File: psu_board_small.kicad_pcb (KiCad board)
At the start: 2 copper layers, 23 parts

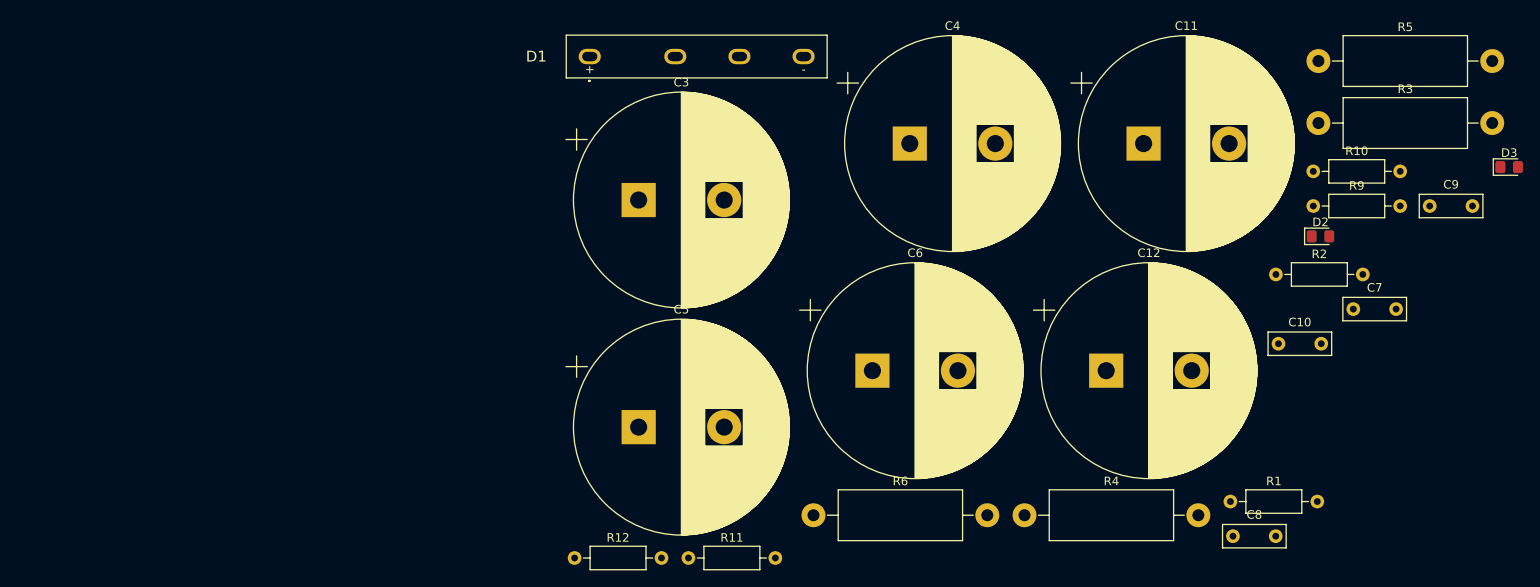
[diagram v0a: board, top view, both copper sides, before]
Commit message: finished pcb layout
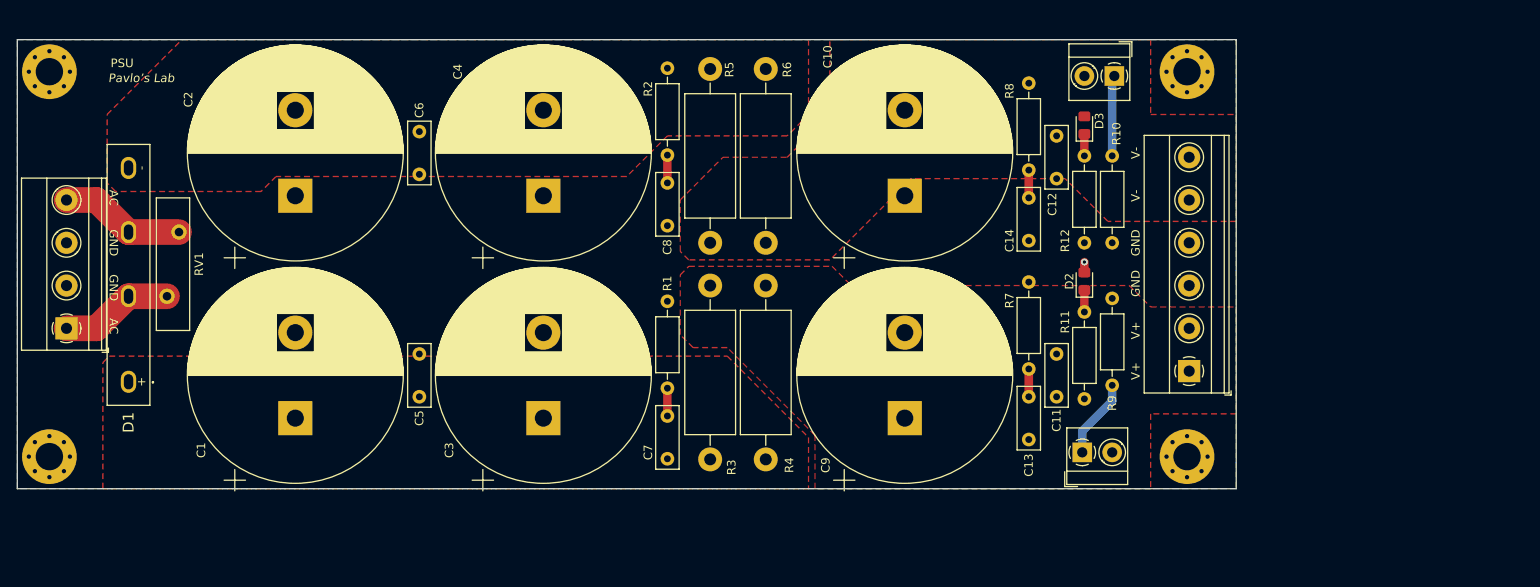
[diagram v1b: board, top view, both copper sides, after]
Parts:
- added C11: 100n, Capacitor_THT:C_Rect_L7.2mm_W2.5mm_P5.00mm_FKS2_FKP2_MKS2_MKP2, F.Cu at (144.0, 108.0)
- added C12: 100n, Capacitor_THT:C_Rect_L7.2mm_W2.5mm_P5.00mm_FKS2_FKP2_MKS2_MKP2, F.Cu at (144.0, 82.5)
- added C13: 100n, Capacitor_THT:C_Rect_L7.2mm_W2.5mm_P5.00mm_FKS2_FKP2_MKS2_MKP2, F.Cu at (140.8, 113.0)
- added C14: 100n, Capacitor_THT:C_Rect_L7.2mm_W2.5mm_P5.00mm_FKS2_FKP2_MKS2_MKP2, F.Cu at (140.8, 89.8)
- added H1: MountingHole, MountingHole:MountingHole_3.2mm_M3_Pad_Via, F.Cu at (26.2, 115.0)
- added H2: MountingHole, MountingHole:MountingHole_3.2mm_M3_Pad_Via, F.Cu at (26.2, 70.0)
- added H3: MountingHole, MountingHole:MountingHole_3.2mm_M3_Pad_Via, F.Cu at (159.2, 70.0)
- added H4: MountingHole, MountingHole:MountingHole_3.2mm_M3_Pad_Via, F.Cu at (159.2, 115.0)
- added J1: AC, TerminalBlock_Phoenix:TerminalBlock_Phoenix_MKDS-1,5-4_1x04_P5.00mm_Horizontal, F.Cu at (28.2, 100.0)
- added J2: LED, TerminalBlock_MetzConnect:TerminalBlock_MetzConnect_Type059_RT06302HBWC_1x02_P3.50mm_Horizontal, F.Cu at (147.0, 114.5)
- added J3: LED, TerminalBlock_MetzConnect:TerminalBlock_MetzConnect_Type059_RT06302HBWC_1x02_P3.50mm_Horizontal, F.Cu at (150.8, 70.5)
- added J4: DC, TerminalBlock_Phoenix:TerminalBlock_Phoenix_MKDS-1,5-6_1x06_P5.00mm_Horizontal, F.Cu at (159.5, 105.0)
- added R7: 10R, Resistor_THT:R_Axial_DIN0207_L6.3mm_D2.5mm_P10.16mm_Horizontal, F.Cu at (140.8, 104.8)
- added R8: 10R, Resistor_THT:R_Axial_DIN0207_L6.3mm_D2.5mm_P10.16mm_Horizontal, F.Cu at (140.8, 81.5)
- added RV1: MOV-14D101KTR, Varistor:RV_Disc_D15.5mm_W3.9mm_P7.5mm, F.Cu at (40.0, 96.2)
- moved C5 109.7 mm to (69.5, 108.0), turned to 90 degrees
- moved C6 104.1 mm to (69.5, 82.0), turned to 90 degrees
- moved C7 93.9 mm to (98.5, 115.2), turned to 90 degrees
- moved R5 74.2 mm to (103.5, 90.0), turned to 90 degrees
- moved R3 73.6 mm to (103.5, 95.0), turned to 270 degrees
- moved C8 72.8 mm to (98.5, 88.0), turned to 90 degrees
- moved R2 72.5 mm to (98.5, 79.8), turned to 90 degrees
- moved C2 72.1 mm to (55.0, 84.5), turned to 90 degrees
- moved D1 71.9 mm to (35.5, 92.5), turned to 90 degrees
- moved R12 70.1 mm to (147.2, 90.0), turned to 90 degrees
- moved R1 67.1 mm to (98.5, 107.0), turned to 90 degrees
- moved D3 49.9 mm to (147.2, 76.2), turned to 90 degrees
- moved R11 49.9 mm to (147.2, 108.2), turned to 90 degrees
- moved C1 47.6 mm to (55.0, 110.5), turned to 90 degrees
- moved C4 43.6 mm to (84.0, 84.5), turned to 90 degrees
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- renumbered C3 to C1, C12 to C10, C4 to C2, C5 to C3, C6 to C4, C7 to C5, C8 to C6, C9 to C7, C10 to C8, C11 to C9
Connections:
- D1 pad 2: (no net) -> /AC1
- D1 pad 3: (no net) -> /AC4
- R10 pad 2: (no net) -> Net-(J3-Pad1)
- R9 pad 2: (no net) -> Net-(J2-Pad1)
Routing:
- net /AC4: track 0.00 -> 14.7 mm
- net /AC1: track 0.00 -> 13.3 mm
- net Net-(J3-Pad1): track 0.00 -> 9.44 mm
- net Net-(J2-Pad1): track 0.00 -> 9.29 mm
- net Net-(C8-Pad2): track 0.00 -> 3.25 mm
- net Net-(C7-Pad2): track 0.00 -> 3.25 mm
- net Net-(C14-Pad2): track 0.00 -> 3.25 mm
- net Net-(C13-Pad2): track 0.00 -> 3.25 mm
- net Net-(D3-Pad1): track 0.00 -> 2.56 mm
- net Net-(D2-Pad1): track 0.00 -> 2.56 mm
- net GND: track 0.00 -> 1.22 mm, vias 0 -> 1
- added copper zone on F.Cu, net /OV+
- added copper zone on F.Cu, net /OV-
- added copper zone on F.Cu, net /RV+
- added copper zone on F.Cu, net /RV-
- added copper zone on B.Cu, net GND
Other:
- board outline added: 142.5 x 52.5 mm
- board text added: "AC"
- board text added: "GND"
- board text added: "July 2023"
- board text added: "PSU"
- board text added: "Pavlo’s Lab"
- board text added: "Rev1.0"
- board text added: "V+"
- board text added: "V-"

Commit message: updated rev2
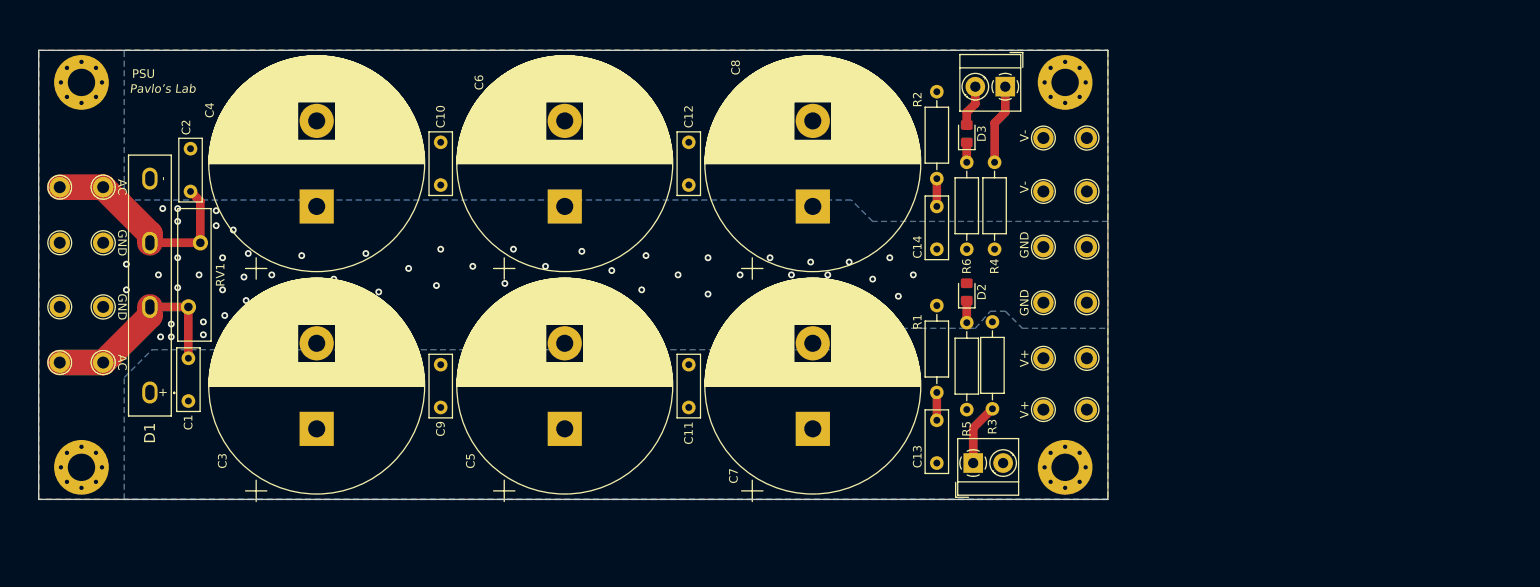
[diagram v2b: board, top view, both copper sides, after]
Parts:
- removed the C13 at (140.8, 113.0)
- removed the C14 at (140.8, 89.8)
- removed the R3 at (103.5, 95.0)
- removed the R4 at (110.0, 95.0)
- removed the R5 at (103.5, 90.0)
- removed the R6 at (110.0, 90.0)
- removed R7, R8: 10R, Resistor_THT:R_Axial_DIN0207_L6.3mm_D2.5mm_P10.16mm_Horizontal
- added C1: 100n, Capacitor_THT:C_Rect_L7.2mm_W2.5mm_P5.00mm_FKS2_FKP2_MKS2_MKP2, F.Cu at (42.5, 103.5)
- added C2: 100n, Capacitor_THT:C_Rect_L7.2mm_W2.5mm_P5.00mm_FKS2_FKP2_MKS2_MKP2, F.Cu at (42.8, 79.0)
- added J10: GND, local_footprints_lib:Terminal_.25_PCB_TAB_TE_Connectivity_P5.08mm_, F.Cu at (145.0, 97.0)
- added J11: V-, local_footprints_lib:Terminal_.25_PCB_TAB_TE_Connectivity_P5.08mm_, F.Cu at (145.0, 77.8)
- added J12: V-, local_footprints_lib:Terminal_.25_PCB_TAB_TE_Connectivity_P5.08mm_, F.Cu at (145.0, 84.0)
- added J2: GND2, local_footprints_lib:Terminal_.25_PCB_TAB_TE_Connectivity_P5.08mm_, F.Cu at (30.0, 90.0)
- added J3: GND3, local_footprints_lib:Terminal_.25_PCB_TAB_TE_Connectivity_P5.08mm_, F.Cu at (30.0, 97.5)
- added J7: V+, local_footprints_lib:Terminal_.25_PCB_TAB_TE_Connectivity_P5.08mm_, F.Cu at (145.0, 109.5)
- added J8: V+, local_footprints_lib:Terminal_.25_PCB_TAB_TE_Connectivity_P5.08mm_, F.Cu at (145.0, 103.5)
- added J9: GND, local_footprints_lib:Terminal_.25_PCB_TAB_TE_Connectivity_P5.08mm_, F.Cu at (145.0, 90.5)
- J1: value AC -> AC1; footprint TerminalBlock_Phoenix:TerminalBlock_Phoenix_MKDS-1,5-4_1x04_P5.00mm_Horizontal -> local_footprints_lib:Terminal_.25_PCB_TAB_TE_Connectivity_P5.08mm_
- J4: value DC -> AC4; footprint TerminalBlock_Phoenix:TerminalBlock_Phoenix_MKDS-1,5-6_1x06_P5.00mm_Horizontal -> local_footprints_lib:Terminal_.25_PCB_TAB_TE_Connectivity_P5.08mm_
- moved J4 131.3 mm to (30.0, 83.5), turned to 0 degrees
- moved C11 43.0 mm to (101.0, 109.2)
- moved C12 43.0 mm to (101.0, 83.2)
- moved C14 31.6 mm to (130.0, 90.8)
- moved R2 31.6 mm to (130.0, 82.5)
- moved C13 31.5 mm to (130.0, 115.8)
- moved R1 31.5 mm to (130.0, 107.5)
- moved H3 14.3 mm to (145.0, 71.2)
- moved H4 14.3 mm to (145.0, 116.2)
- moved R3 14.3 mm to (136.5, 99.2)
- moved D2 13.8 mm to (133.5, 95.8)
- moved R5 13.8 mm to (133.5, 109.5)
- moved D3 13.8 mm to (133.5, 77.2)
- moved R4 13.8 mm to (136.8, 90.8)
- moved R6 13.8 mm to (133.5, 90.8)
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- renumbered C6 to C10, C7 to C13, C8 to C14, C1 to C3, C2 to C4, C3 to C5, C4 to C6, C9 to C7, C10 to C8, C5 to C9, J2 to J5, J3 to J6, R9 to R3, R10 to R4, R11 to R5, R12 to R6
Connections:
- C10 pad 2: /RV- -> /V-
- C11 pad 1: /OV+ -> /V+
- C12 pad 2: /OV- -> /V-
- C13 pad 1: /RV+ -> /V+
- C3 pad 1: /RV+ -> /V+
- C4 pad 2: /RV- -> /V-
- C5 pad 1: /RV+ -> /V+
- C6 pad 2: /RV- -> /V-
- C7 pad 1: /OV+ -> /V+
- C8 pad 2: /OV- -> /V-
- C9 pad 1: /RV+ -> /V+
- D1 pad 1: /RV+ -> /V+
- D1 pad 4: /RV- -> /V-
- D3 pad 2: /OV- -> /V-
- J4 pad 1: /OV+ -> /AC4
- J6 pad 2: /OV- -> /V-
- R2 pad 2: /RV- -> /V-
- R3 pad 1: /OV+ -> /V+
- R5 pad 1: /OV+ -> /V+
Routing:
- net /AC4: track 14.7 -> 26.2 mm
- net /AC1: track 13.3 -> 24.3 mm
- net /V-: track 0.00 -> 4.89 mm
- net Net-(C14-Pad2) (its old number): track 3.25 -> 0.00 mm
- net Net-(C13-Pad2) (its old number): track 3.25 -> 0.00 mm
- net Net-(J5-Pad1): track 9.29 -> 7.27 mm
- net GND: track 1.22 -> 0.00 mm, vias 1 -> 57
- added copper zone on B.Cu, net /V+
- added copper zone on B.Cu, net /V-
- added copper zone on F.Cu, net GND
- removed copper zone on F.Cu, net /OV+
- removed copper zone on F.Cu, net /OV-
- removed copper zone on F.Cu, net /RV+
- removed copper zone on F.Cu, net /RV-
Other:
- board size 142.5 x 52.5 mm -> 125 x 52.5 mm
- board text added: "December 2023"
- board text added: "Rev2.0"
- board text removed: "July 2023"
- board text removed: "Rev1.0"
